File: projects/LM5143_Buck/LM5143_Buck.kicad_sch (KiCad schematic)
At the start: 91 parts, among them J1 Bat In, J2 24V Out, J3 I2C Socket, J4 I2C Socket, Q1 IGC025S08S1, Q2 IGC025S08S1, Q3 IGC025S08S1, Q4 IGC025S08S1, SW1 Addr_Switch, SW2 Addr_Switch, U2 TLV74033, U3 INA226

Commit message: Change switch orientation, update XT60 name
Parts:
- J1, J2: footprint footprints:XT60PW-F -> footprints:XT60PW
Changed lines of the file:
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@@
 			)
 		)
-		(property "Footprint" "footprints:XT60PW-F"
+		(property "Footprint" "footprints:XT60PW"
 			(at 194.31 138.43 0)
 			(effects
@@
 			)
 		)
-		(property "Footprint" "footprints:XT60PW-F"
+		(property "Footprint" "footprints:XT60PW"
 			(at 194.31 149.86 0)
 			(effects

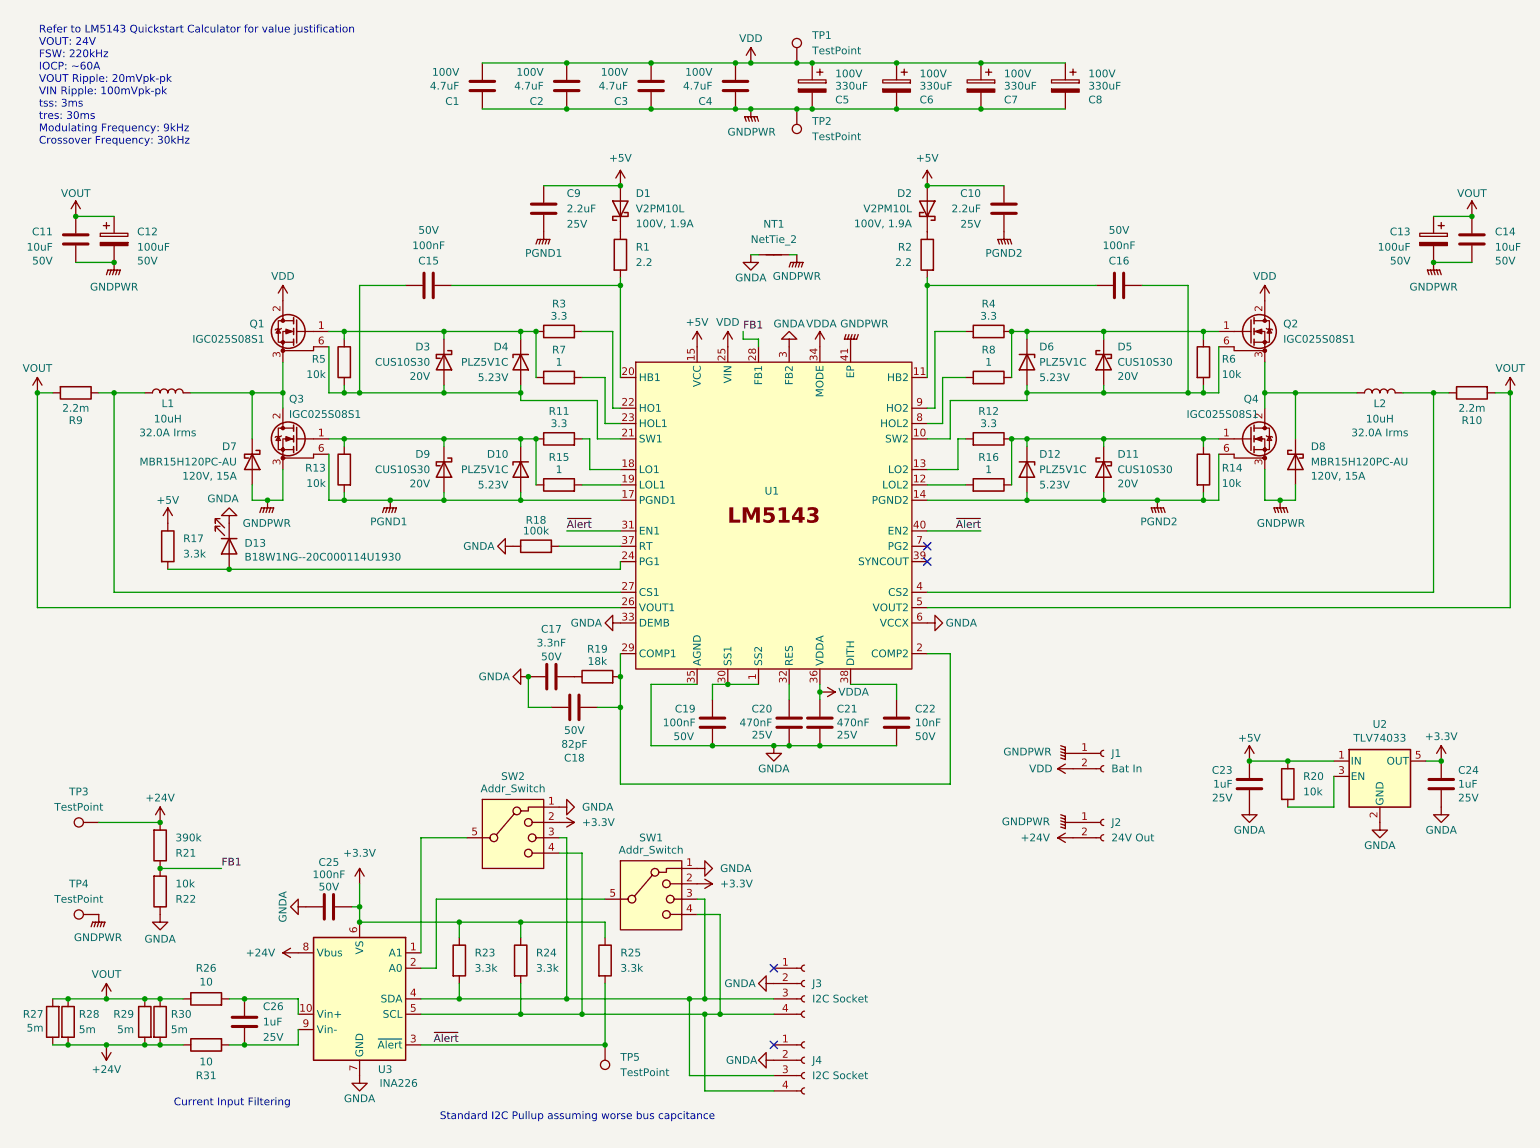
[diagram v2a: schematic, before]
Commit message: New Schematic
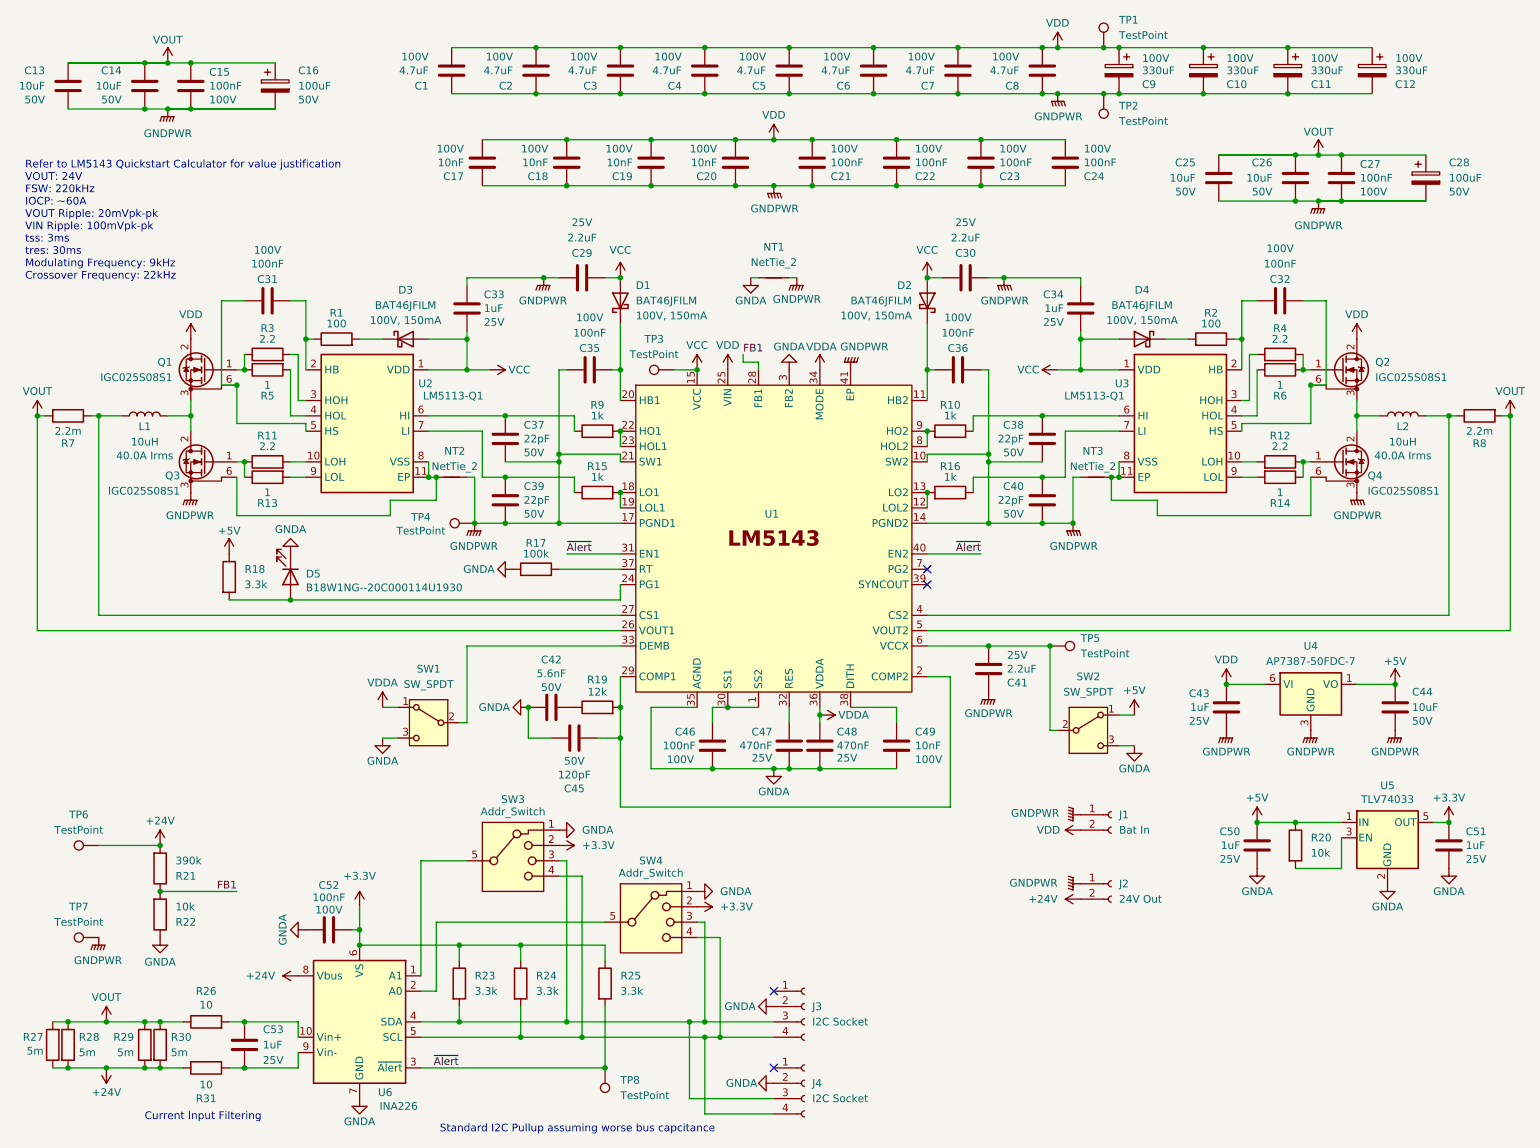
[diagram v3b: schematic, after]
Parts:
- removed C10, C9: 2.2uF, Capacitor_SMD:C_0805_2012Metric, symbol Device:C
- removed C13: 100uF, Capacitor_THT:CP_Radial_D8.0mm_P3.50mm, symbol Device:C_Polarized
- removed C14: 10uF, Capacitor_SMD:C_1210_3225Metric, symbol Device:C
- removed C16: 100nF, Capacitor_SMD:C_0603_1608Metric, symbol Device:C
- removed D10, D12, D4, D6: PLZ5V1C, footprints:D_MicroSMF, symbol Device:D_Zener
- removed D11, D5, D9: CUS10S30, Diode_SMD:D_SOD-323_HandSoldering, symbol Device:D_Schottky
- removed D7, D8: MBR15H120PC-AU, Package_TO_SOT_SMD:TO-277A, symbol Device:D_Schottky
- removed R7: 1, Resistor_SMD:R_0603_1608Metric, symbol Device:R
- added C1, C2, C3, C4: 4.7uF, Capacitor_SMD:C_1210_3225Metric, symbol Device:C
- added C13, C25, C26, C44: 10uF, Capacitor_SMD:C_1210_3225Metric, symbol Device:C
- added C15, C21, C22, C23, C24, C27, C31, C32, C36: 100nF, Capacitor_SMD:C_0603_1608Metric, symbol Device:C
- added C17, C18, C19, C20: 10nF, Capacitor_SMD:C_0603_1608Metric, symbol Device:C
- added C28: 100uF, Capacitor_THT:CP_Radial_D8.0mm_P3.50mm, symbol Device:C_Polarized
- added C29, C30, C41: 2.2uF, Capacitor_SMD:C_0805_2012Metric, symbol Device:C
- added C33, C34, C43: 1uF, Capacitor_SMD:C_0603_1608Metric, symbol Device:C
- added C37, C38, C39, C40: 22pF, Capacitor_SMD:C_0603_1608Metric, symbol Device:C
- added D4: BAT46JFILM, footprints:D_SOD-323_Alt, symbol Device:D_Schottky
- added NT2, NT3: NetTie_2, footprints:NetTie-2_SMD_Pad0.25mm, symbol Device:NetTie_2
- added R9: 1k, Resistor_SMD:R_0603_1608Metric, symbol Device:R
- added SW1, SW2: SW_SPDT, footprints:SLW-865144-2A-N-SMT-TR, symbol Switch:SW_SPDT
- added TP3, TP4: TestPoint, TestPoint:TestPoint_Keystone_5000-5004_Miniature, symbol Connector:TestPoint
- added TP5: TestPoint, TestPoint:TestPoint_Pad_D2.0mm, symbol Connector:TestPoint
- added U2, U3: LM5113-Q1, Package_SON:WSON-10-1EP_4x4mm_P0.8mm_EP2.6x3mm_ThermalVias, symbol symbols:LM5113-Q1
- added U4: AP7387-50FDC-7, Package_DFN_QFN:DFN-6-1EP_2x2mm_P0.65mm_EP1.01x1.7mm, symbol Regulator_Linear:AP7370-50FDC
- C35: renamed from C15; Voltage 50V -> 100V
- C42: renamed from C17; value 3.3nF -> 5.6nF
- C45: renamed from C18; value 82pF -> 120pF
- C46: renamed from C19; Voltage 50V -> 100V
- C49: renamed from C22; Voltage 50V -> 100V
- C52: renamed from C25; Voltage 50V -> 100V
- D1, D2: value V2PM10L -> BAT46JFILM; footprint Diode_SMD:D_SMP_DO-220AA -> footprints:D_SOD-323_Alt; Descr 100V, 1.9A -> 100V, 150mA
- D3: value CUS10S30 -> BAT46JFILM; footprint Diode_SMD:D_SOD-323_HandSoldering -> footprints:D_SOD-323_Alt; Descr 20V -> 100V, 150mA
- L1, L2: footprint footprints:ER26A -> footprints:CPQ2620H; Irms 32.0A Irms -> 40.0A Irms
- R1, R2: value 2.2 -> 100
- R10: value 2.2m -> 1k; footprint footprints:ASR2512 -> Resistor_SMD:R_0603_1608Metric
- R11, R12, R3, R4: value 3.3 -> 2.2
- R13, R14, R5, R6: value 10k -> 1
- R15, R16: value 1 -> 1k
- R19: value 18k -> 12k
- R8: value 1 -> 2.2m; footprint Resistor_SMD:R_0603_1608Metric -> footprints:ASR2512
- renumbered C6 to C10, C7 to C11, C8 to C12, C11 to C14, C12 to C16, C20 to C47, C21 to C48, C1 to C5, C23 to C50, C24 to C51, C26 to C53, C2 to C6, C3 to C7, C4 to C8, C5 to C9, D13 to D5, R18 to R17, R17 to R18, R9 to R7, SW2 to SW3, SW1 to SW4, TP3 to TP6, TP4 to TP7, TP5 to TP8, U2 to U5, U3 to U6
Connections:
- net +5V: now also C44.1, SW2.1 (A), U4.1 (VO); no longer D1.2 (A), D2.2 (A), U1.15 (VCC), U1.16 (VCC)
- net GNDA: now also SW1.3 (C), SW2.3 (C); no longer U1.33 (DEMB), U1.6 (VCCX)
- net VDD: now also C1.2, C17.2, C18.2, C19.2, C2.2, C20.2, C21.2, C22.2, C23.2, C24.2, C3.2, C4.2, C43.1, U4.6 (VI)
- net VDDA: now also SW1.1 (A)
- net VOUT: now also R8.2, C13.1, C15.1, C25.1, C26.1, C27.1, C28.1; no longer R10.2
- net at Q4.1 (G), R12.1, R14.1: no longer R16.1
- net at Q2.3 (S), Q2.5 (S), Q4.2 (D)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: now also L2.2; no longer L2.1
- net at Q1.1 (G), R3.1, R5.1: no longer D3.1 (K)
- net at Q3.1 (G), R11.1, R13.1: no longer R15.1
- net at U1.22 (HO1): now also U1.23 (HOL1), R9.2; no longer R3.2
- net at Q2.1 (G), R4.1, R6.1: no longer R8.1
- net at D2.1 (K): now also U1.11 (HB2), C36.2; no longer R2.1
- net at R2.2: now also D4.1 (K); no longer U1.11 (HB2)
- net at R16.2, U1.12 (LOL2): now also U1.13 (LO2)
- net at R12.2: now also U3.10 (LOH); no longer U1.13 (LO2)
- net at U1.18 (LO1): now also R15.2, U1.19 (LOL1); no longer R11.2
- net at C35.2, U1.20 (HB1): now also D1.1 (K); no longer R1.2
- net at U1.8 (HOL2): now also R10.2, U1.9 (HO2); no longer R8.2
- net at R4.2: now also U3.3 (HOH); no longer U1.9 (HO2)
- net at R1.1: now also C31.2, U2.2 (HB); no longer D1.1 (K)
- net GNDPWR renamed GND
- net GND: now also C35.1, U1.10 (SW2), U1.14 (PGND2), U1.17 (PGND1), U1.21 (SW1), C1.1, C13.2, C15.2, C17.1, C18.1, C19.1, C2.1, C20.1, C21.1, C22.1, C23.1, C24.1, C25.2, C26.2, C27.2, C28.2, C29.1, C3.1, C30.1, C33.1, C34.1, C36.1, C37.2, C38.2, C39.2, C4.1, C40.2, C41.1, C43.2, C44.2, NT2.2, NT3.2, TP4.1, U4.2 (GND), U4.3 (GND), U4.4 (GND), U4.5 (GND), U4.7 (GND)
- removed net PGND1: Q3.6 (DS), R13.2, U1.17 (PGND1)
- removed net PGND2: Q4.6 (DS), R14.2, U1.14 (PGND2)
- new net: D3.1 (K), R1.2
- new net: C41.2, SW2.2 (B), TP5.1, U1.6 (VCCX)
- new net: SW1.2 (B), U1.33 (DEMB)
- new net: L2.1, R8.1, U1.4 (CS2)
- new net: C38.1, R10.1, U3.6 (HI)
- new net: C31.1, Q1.6 (DS), U2.5 (HS)
- new net: R11.2, U2.10 (LOH)
- new net: R3.2, U2.3 (HOH)
- new net: C32.1, Q2.6 (DS), U3.5 (HS)
- new net: C37.1, R9.1, U2.6 (HI)
- new net: C40.1, R16.1, U3.7 (LI)
- new net: NT2.1, Q3.6 (DS), U2.11 (EP), U2.8 (VSS)
- new net: R5.2, U2.4 (HOL)
- new net: C39.1, R15.1, U2.7 (LI)
- new net: R13.2, U2.9 (LOL)
- new net: NT3.1, Q4.6 (DS), U3.11 (EP), U3.8 (VSS)
- new net: C32.2, R2.1, U3.2 (HB)
- new net: R6.2, U3.4 (HOL)
- new net: R14.2, U3.9 (LOL)
- new net VCC: C29.2, C30.2, C33.2, C34.2, D1.2 (A), D2.2 (A), D3.2 (A), D4.2 (A), TP3.1, U1.15 (VCC), U1.16 (VCC), U2.1 (VDD), U3.1 (VDD)
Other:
- note added: "Refer to LM5143 Quickstart Calculator for value justification VOUT: 24V FSW: 220kHz IOCP: ~60A VOUT Ripple: 20mVpk-pk VIN Ripple: 100mVpk-pk tss: 3ms tres: 30ms Modulating Frequency: 9kHz Crossover Frequency: 22kHz"
- note removed: "Refer to LM5143 Quickstart Calculator for value justification VOUT: 24V FSW: 220kHz IOCP: ~60A VOUT Ripple: 20mVpk-pk VIN Ripple: 100mVpk-pk tss: 3ms tres: 30ms Modulating Frequency: 9kHz Crossover Frequency: 30kHz"
- moved on the sheet: C10, C11, C12, C14, C16, C35, C42, C45, C46, C47, C48, C49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
